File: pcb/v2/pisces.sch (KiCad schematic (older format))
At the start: 54 parts, among them J1 USB_B_Micro, J2 AudioJack4, SW1 SW_PUSH, SW10 SW_PUSH, SW11 SW_PUSH, SW12 SW_PUSH, SW13 SW_PUSH, SW14 SW_PUSH, SW15 SW_PUSH, SW16 SW_PUSH, SW17 SW_PUSH, SW18 SW_PUSH, SW19 SW_PUSH, SW2 SW_PUSH, SW3 SW_PUSH, SW4 SW_PUSH, SW5 SW_PUSH, SW6 SW_PUSH, SW7 SW_PUSH, SW8 SW_PUSH, SW9 SW_PUSH, U1 ATmega32U2-AU, Y1 Crystal_GND24_Small

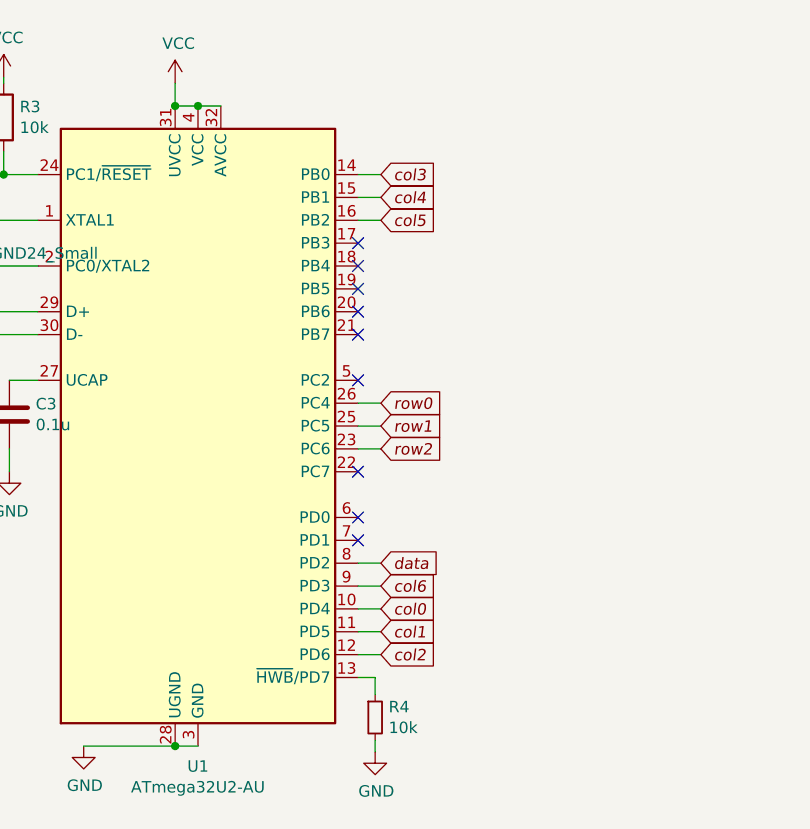
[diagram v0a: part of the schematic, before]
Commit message: Done with routing
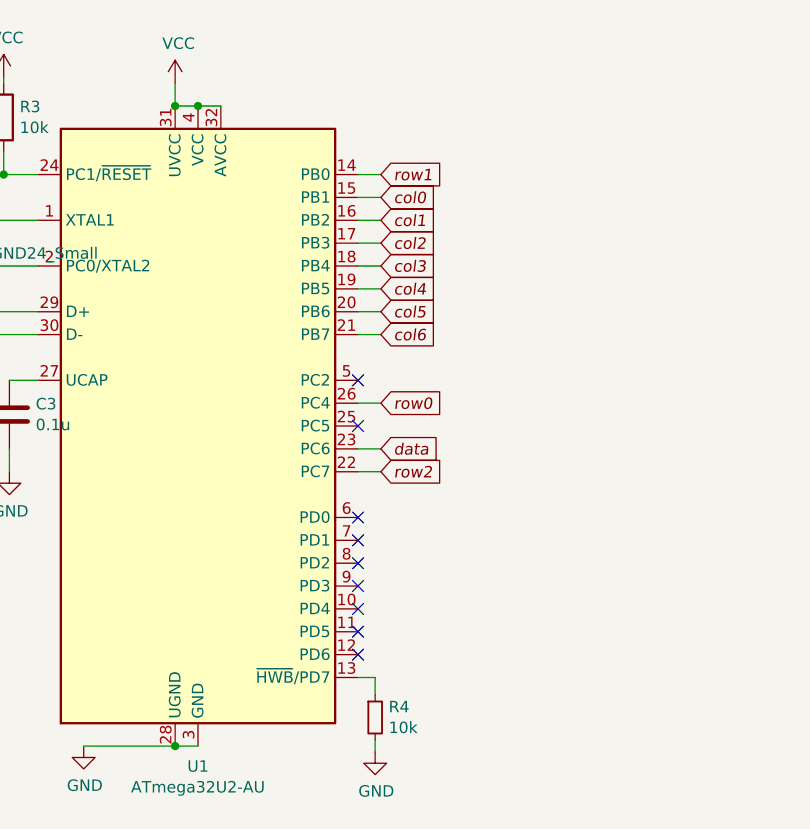
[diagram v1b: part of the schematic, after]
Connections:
- net col0: now also U1.15 (PB1); no longer U1.10 (PD4)
- net col1: now also U1.16 (PB2); no longer U1.11 (PD5)
- net col2: now also U1.17 (PB3); no longer U1.12 (PD6)
- net col3: now also U1.18 (PB4); no longer U1.14 (PB0)
- net col4: now also U1.19 (PB5); no longer U1.15 (PB1)
- net col5: now also U1.20 (PB6); no longer U1.16 (PB2)
- net col6: now also U1.21 (PB7); no longer U1.9 (PD3)
- net data: now also U1.23 (PC6); no longer U1.8 (PD2)
- net row1: now also U1.14 (PB0); no longer U1.25 (PC5)
- net row2: now also U1.22 (PC7); no longer U1.23 (PC6)
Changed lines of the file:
@@
 Wire Wire Line
 	9275 925  9275 2550
-Text GLabel 6225 5925 2    50   Input Italic 0
+Text GLabel 6225 4825 2    50   Input Italic 0
 col6
 Text Notes 3175 3175 2    50   Italic 0
@@
 Wire Wire Line
 	2900 3575 2900 3475
-Text GLabel 6225 5825 2    50   Input Italic 0
+Text GLabel 6225 5325 2    50   Input Italic 0
 data
 $Comp
@@
 Text GLabel 6225 5125 2    50   Input Italic 0
 row0
-Text GLabel 6225 5225 2    50   Input Italic 0
+Text GLabel 6225 4125 2    50   Input Italic 0
 row1
-Text GLabel 6225 5325 2    50   Input Italic 0
+Text GLabel 6225 5425 2    50   Input Italic 0
 row2
-Text GLabel 6225 6025 2    50   Input Italic 0
+Text GLabel 6225 4225 2    50   Input Italic 0
 col0
-Text GLabel 6225 6125 2    50   Input Italic 0
+Text GLabel 6225 4325 2    50   Input Italic 0
 col1
-Text GLabel 6225 6225 2    50   Input Italic 0
+Text GLabel 6225 4425 2    50   Input Italic 0
 col2
-Text GLabel 6225 4125 2    50   Input Italic 0
+Text GLabel 6225 4525 2    50   Input Italic 0
 col3
-Text GLabel 6225 4225 2    50   Input Italic 0
+Text GLabel 6225 4625 2    50   Input Italic 0
 col4
-Text GLabel 6225 4325 2    50   Input Italic 0
+Text GLabel 6225 4725 2    50   Input Italic 0
 col5
 $Comp
@@
 	6125 5125 6225 5125
 Wire Wire Line
-	6125 5225 6225 5225
-Wire Wire Line
-	6125 5325 6225 5325
-Wire Wire Line
 	4575 4125 4725 4125
-NoConn ~ 6125 5425
 NoConn ~ 6125 5625
 $Comp
@@
 Wire Wire Line
 	950  6600 950  6800
-NoConn ~ 6125 4625
 $Comp
 L Device:R_Small R4
@@
 Wire Wire Line
 	6200 6600 6200 6650
-Wire Wire Line
-	6125 4325 6225 4325
-Wire Wire Line
-	6125 4225 6225 4225
-Wire Wire Line
-	6125 4125 6225 4125
-Wire Wire Line
-	6125 6225 6225 6225
-Wire Wire Line
-	6125 6025 6225 6025
-Wire Wire Line
-	6125 6125 6225 6125
-NoConn ~ 6125 4425
-NoConn ~ 6125 4525
-NoConn ~ 6125 4725
-NoConn ~ 6125 4825
 NoConn ~ 6125 5025
 NoConn ~ 6125 5725
-Wire Wire Line
-	6125 5925 6225 5925
-Wire Wire Line
-	6125 5825 6225 5825
 Text GLabel 8400 925  1    50   Input Italic 0
 col5
@@
 	1    0    0    -1
 $EndComp
+Wire Wire Line
+	6125 5325 6225 5325
+Wire Wire Line
+	6125 5425 6225 5425
+NoConn ~ 6125 5825
+Wire Wire Line
+	6125 4825 6225 4825
+NoConn ~ 6125 5925
+Wire Wire Line
+	6125 4725 6225 4725
+Wire Wire Line
+	6125 4625 6225 4625
+Wire Wire Line
+	6125 4525 6225 4525
+Wire Wire Line
+	6125 4425 6225 4425
+NoConn ~ 6125 6225
+Wire Wire Line
+	6125 4325 6225 4325
+NoConn ~ 6125 6125
+NoConn ~ 6125 6025
+Wire Wire Line
+	6125 4225 6225 4225
+Wire Wire Line
+	6125 4125 6225 4125
+NoConn ~ 6125 5225
 $EndSCHEMATC
